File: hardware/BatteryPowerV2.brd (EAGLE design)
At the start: 47 x 40.5 mm, 66 parts, among them Q1 IRLML6402, U1 LT1616ES6TRMPBF, U2 LT6106CS5#PBF, U3 LT1616ES6TRMPBF, U4 LT6106CS5#PBF, U5 TCK106AF,LF, U6 TCK106AF,LF

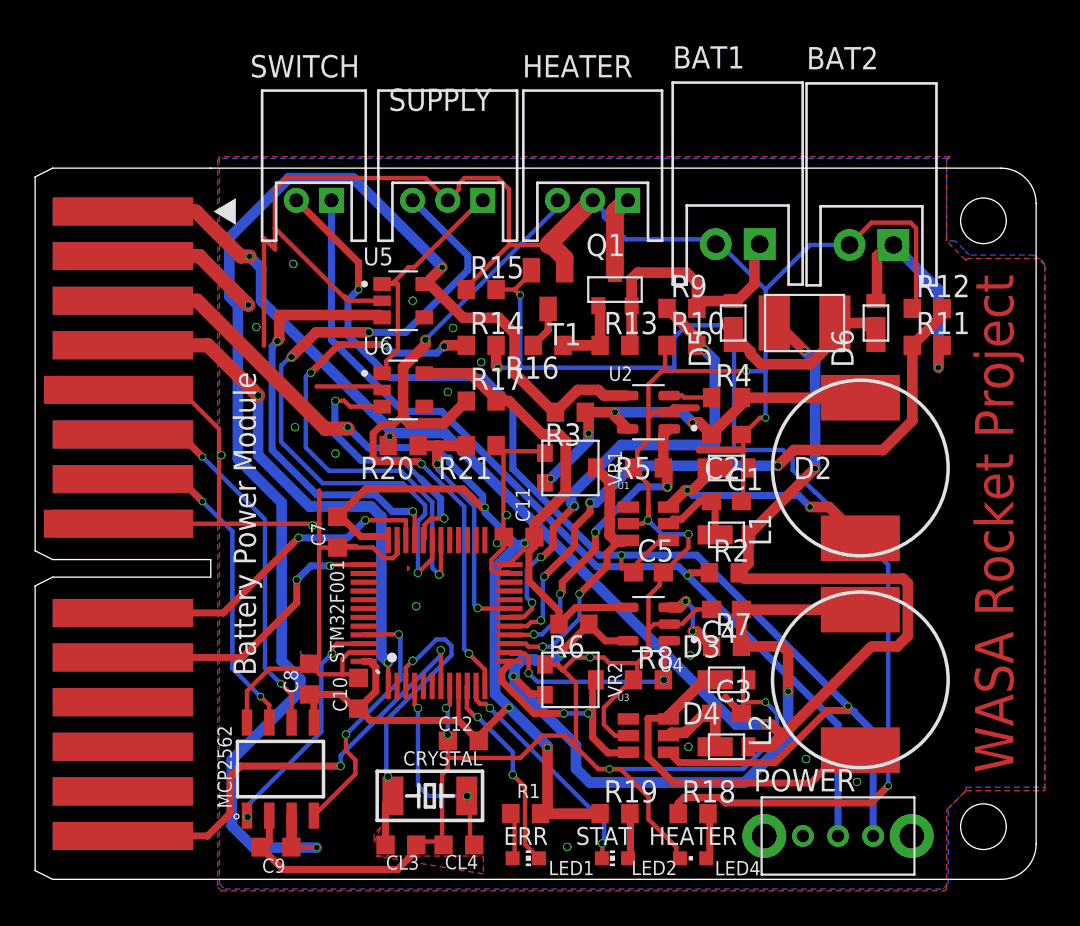
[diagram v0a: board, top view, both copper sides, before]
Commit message: 微調整
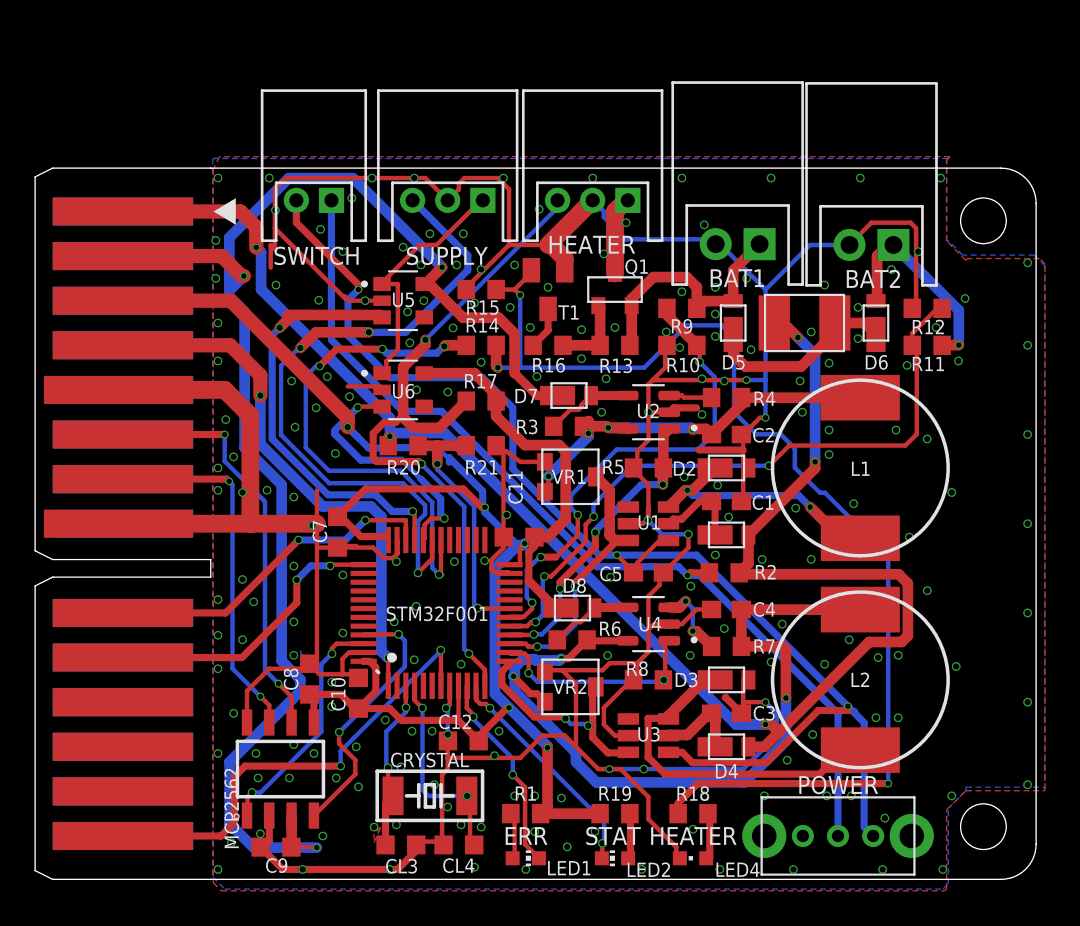
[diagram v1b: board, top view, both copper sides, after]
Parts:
- added D7, D8: CUHS20S30, diodes:CUHS20S30
- moved R6 0.91 mm to (30.6, -6.62)
- moved R3 0.81 mm to (30.4, 5.55)
- moved VR1 0.50 mm to (30.5, 2.67)
- moved VR2 0.40 mm to (30.5, -9.29)
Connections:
- new net VCC': D7.A, R3.2, U2.4
- new net VDD': D8.A, R6.2, U4.4
- net VCC: now also D7.C; no longer R3.2, U2.4
- net VDD: now also D8.C; no longer R6.2, U4.4
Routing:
- net VCC: track 91.0 -> 82.3 mm
- net N$72: track 17.7 -> 9.86 mm
- net GND: track 278.6 -> 273.3 mm, vias 27 -> 204
- net VCC': track 0.00 -> 5.00 mm
- net VDD': track 0.00 -> 4.87 mm
- net 3V3: track 52.6 -> 48.9 mm
- net VDD: track 114.3 -> 110.8 mm
- net N$10: track 68.2 -> 66.2 mm
- net CANH1: track 19.2 -> 20.8 mm
- net CANL1: track 22.3 -> 23.8 mm
- net SUPPLY_3V3: track 17.1 -> 15.9 mm
- net BAT2: track 13.2 -> 12.0 mm
- net BAT1: track 16.0 -> 14.8 mm
- net VPP: track 93.6 -> 94.7 mm
- net N$1: track 13.6 -> 14.7 mm
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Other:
- board text added: "Battery Power Module Ver.2"
- board text added: "WASA Rocket 2023"
- board text removed: "Battery Power Module"
- board text removed: "Designed by @fujiy0, 2019"
- board text removed: "WASA Rocket Project"
